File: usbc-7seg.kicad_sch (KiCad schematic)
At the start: 24 parts, among them J1 USB_C_Receptacle_USB2.0_14P, Q1 AO3400A, Q2 AO3400A, SW1 TS-1088-AR02016, U1 GS2816CX, U2 GS2816CX, U3 CH32V203GxUx, U4 XC6206P332MR-G, Y1 12MHz

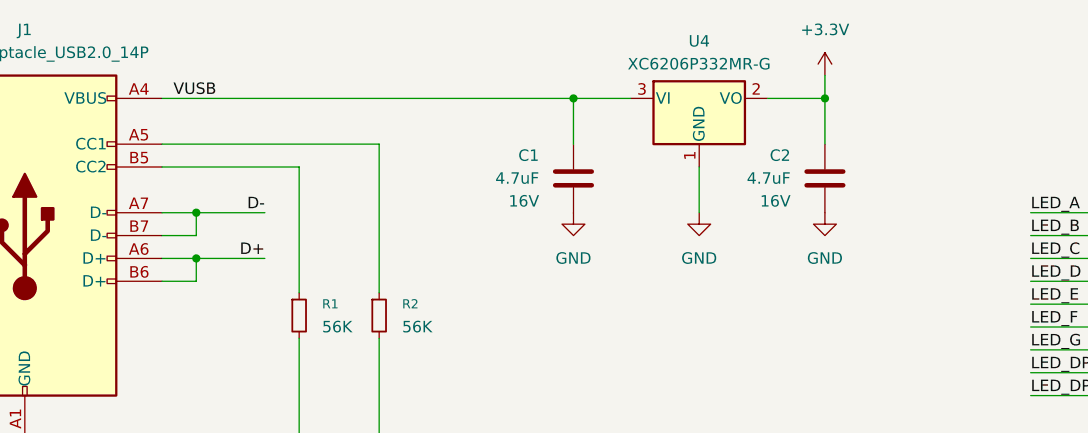
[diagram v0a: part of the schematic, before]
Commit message: Some routing, setup board stackup properly
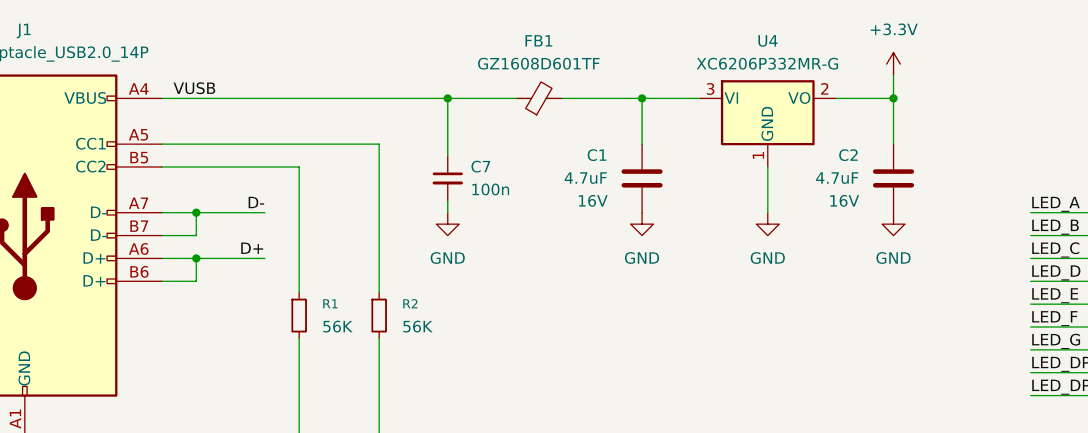
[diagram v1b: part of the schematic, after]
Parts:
- added C7: 100n, Capacitor_SMD:C_0402_1005Metric, symbol Device:C_Small
- added FB1: GZ1608D601TF, Inductor_SMD:L_0603_1608Metric, symbol Device:FerriteBead_Small
- Y1: JLCPCB Part (none) -> C9002
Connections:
- net GND: now also C7.2
- net VUSB: now also C7.1, FB1.1; no longer C1.1, U4.3 (VI)
- new net: C1.1, FB1.2, U4.3 (VI)
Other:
- moved on the sheet: C1, C2, U4
